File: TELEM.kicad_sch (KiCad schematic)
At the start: 11 parts, among them U5 TPS561208DDCR

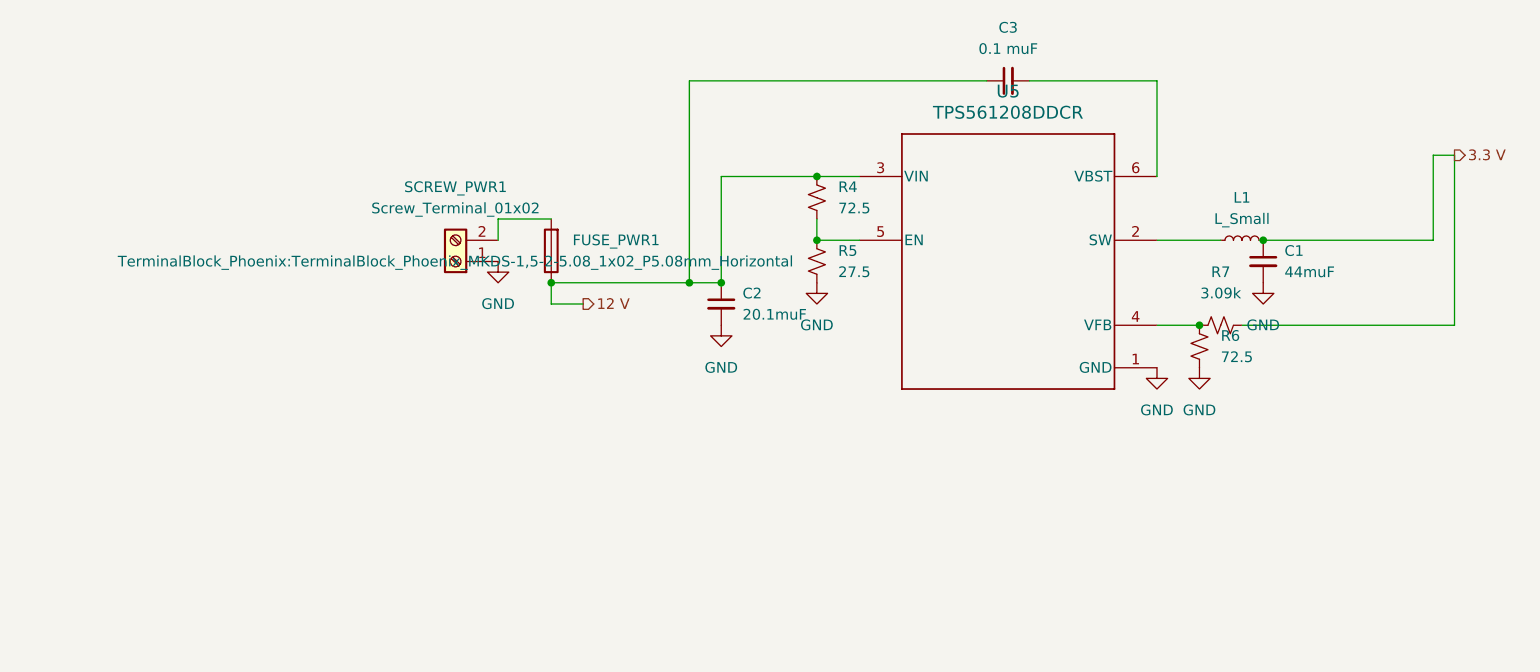
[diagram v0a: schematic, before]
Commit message: Update
Update
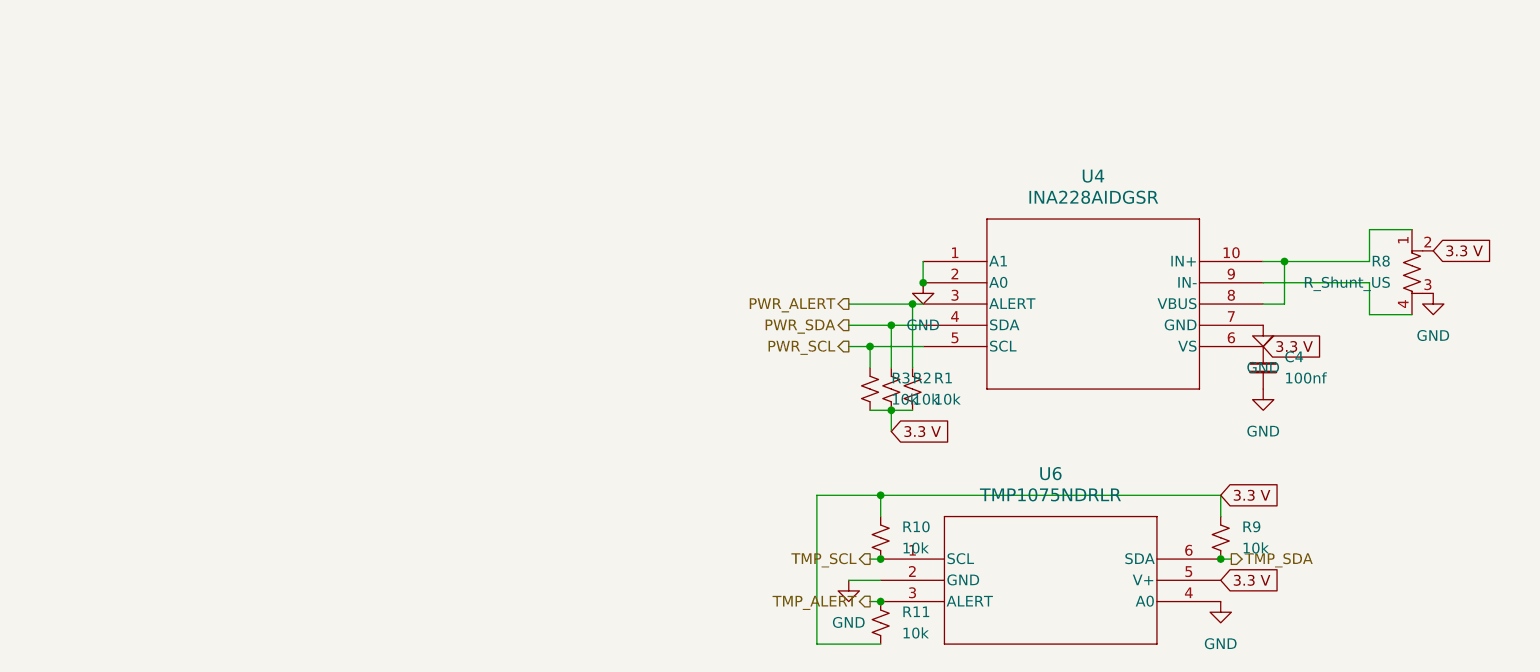
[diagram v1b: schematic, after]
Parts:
- removed C1: 44muF, symbol Device:C_Small
- removed C2: 20.1muF, symbol Device:C_Small
- removed C3: 0.1 muF, symbol Device:C_Small
- removed FUSE_PWR1: 2A 12V PTC fuse, Fuse:Fuse_1812_4532Metric, symbol Device:Fuse
- removed L1: L_Small, symbol Device:L_Small
- removed R4, R6: 72.5, symbol Device:R_Small_US
- removed R5: 27.5, symbol Device:R_Small_US
- removed R7: 3.09k, symbol Device:R_Small_US
- removed SCREW_PWR1: Screw_Terminal_01x02, TerminalBlock_Phoenix:TerminalBlock_Phoenix_MKDS-1,5-2-5.08_1x02_P5.08mm_Horizontal, symbol Connector:Screw_Terminal_01x02
- removed U5: TPS561208DDCR, DDC0006A_N, symbol tpsbuckconv561208:TPS561208DDCR
- added C4: 100nf, symbol Device:C_Small
- added R1, R10, R11, R2, R3, R9: 10k, symbol Device:R_Small_US
- added R8: R_Shunt_US, symbol Device:R_Shunt_US
- added U4: INA228AIDGSR, VSSOP10_DGS_TEX, symbol INA228:INA228AIDGSR
- added U6: TMP1075NDRLR, SOT5X3-6_DRL_TEX, symbol tmpsensor:TMP1075NDRLR
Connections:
- net 3.3 V: now also C4.1, R1.2, R10.1, R11.2, R2.2, R3.2, R8.2, R9.1, U4.6 (VS), U6.5 (V+)
- net GND: now also C4.2, R8.3, U4.1 (A1), U4.2 (A0), U4.7 (GND), U6.2 (GND), U6.4 (A0)
- new net: R8.1, U4.10 (IN+), U4.8 (VBUS)
- new net: R8.4, U4.9 (IN-)
- new net PWR_ALERT: R1.1, U4.3 (ALERT)
- new net PWR_SCL: R3.1, U4.5 (SCL)
- new net PWR_SDA: R2.1, U4.4 (SDA)
- new net TMP_ALERT: R11.1, U6.3 (ALERT)
- new net TMP_SCL: R10.2, U6.1 (SCL)
- new net TMP_SDA: R9.2, U6.6 (SDA)
